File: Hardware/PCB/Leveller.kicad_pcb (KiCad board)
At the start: 2 copper layers, 20 x 48.2 mm, 41 parts, among them J13 Audio to Daisy, connect to J13, J14 Audio from Daisy, connect to 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, J17 Audio output, connect to J16, J18 Audio input, connect to J15, J6 Eurorack_Power, U1 TL074, U2 TL074

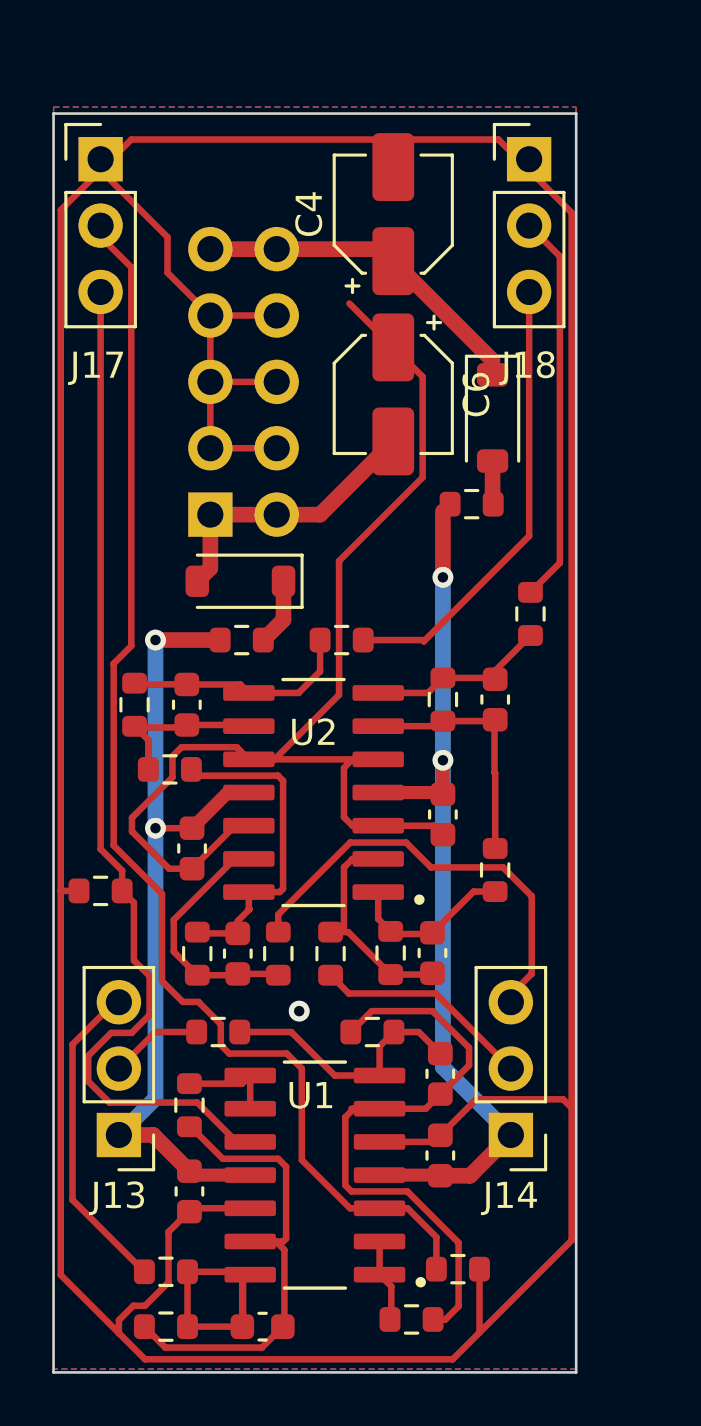
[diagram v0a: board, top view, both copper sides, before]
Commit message: HW 1.0c
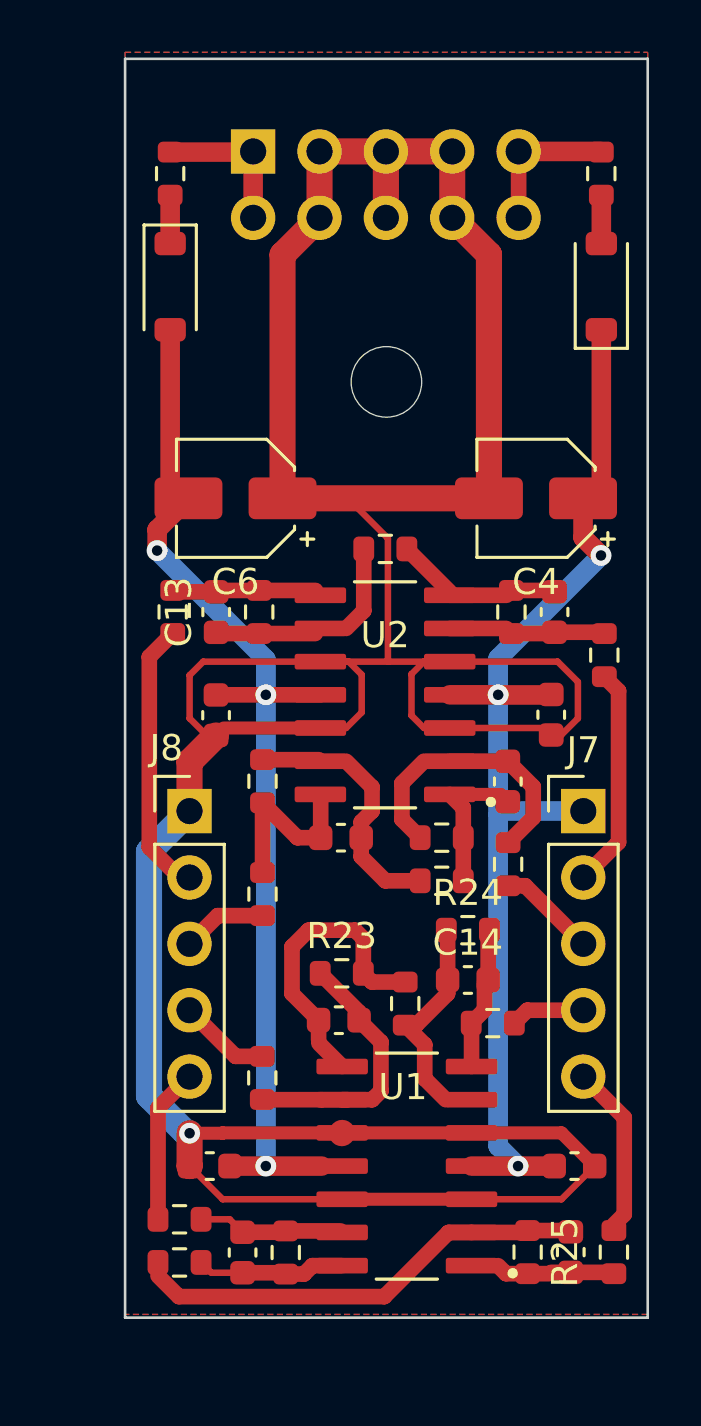
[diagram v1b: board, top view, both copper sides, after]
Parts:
- removed J13: Audio to Daisy, connect to J13, Connector_PinHeader_2.54mm:PinHeader_1x03_P2.54mm_Vertical
- removed J14: Audio from Daisy, connect to J10, Connector_PinHeader_2.54mm:PinHeader_1x03_P2.54mm_Vertical
- removed J17: Audio output, connect to J16, Connector_PinHeader_2.54mm:PinHeader_1x03_P2.54mm_Vertical
- removed J18: Audio input, connect to J15, Connector_PinHeader_2.54mm:PinHeader_1x03_P2.54mm_Vertical
- removed R11: 10K, Resistor_SMD:R_0603_1608Metric
- added C13: 560pF, Capacitor_SMD:C_0603_1608Metric, F.Cu at (58.2, 59.1)
- added C14: 47pF, Capacitor_SMD:C_0603_1608Metric, F.Cu at (67.9, 73.2)
- added J7: Conn_01x05, Connector_PinHeader_2.54mm:PinHeader_1x05_P2.54mm_Vertical, F.Cu at (72.3, 66.7)
- added J8: Conn_01x05, Connector_PinHeader_2.54mm:PinHeader_1x05_P2.54mm_Vertical, F.Cu at (57.2, 66.7)
- added MOUNT1: MountingHole_2.7mm_M2.5, MountingHole:MountingHole_2.7mm_M2.5, F.Cu at (64.7, 50.3)
- added R23: 100K, Resistor_SMD:R_0603_1608Metric, F.Cu at (63.0, 72.9)
- added R24: 100K, Resistor_SMD:R_0603_1608Metric, F.Cu at (67.9, 71.3)
- added R25: 100K, Resistor_SMD:R_0603_1608Metric, F.Cu at (70.1, 83.6)
- C2: value 560pF -> 47pF
- R5: value 2M -> 10K
- R9: value 2M -> 100K
- moved C9 21.1 mm to (59.2, 83.6), turned to 90 degrees
- moved C3 18.9 mm to (63.0, 67.7)
- moved FB1 18.1 mm to (56.5, 42.3), turned to -90 degrees
- moved R12 17.2 mm to (73.4, 83.6), turned to 90 degrees
- moved R9 15.5 mm to (60.9, 83.6), turned to -90 degrees
- moved R18 15.5 mm to (69.4, 68.8)
- moved J6 14.0 mm to (59.6, 41.5), turned to -90 degrees
- moved C7 13.9 mm to (71.2, 59.1)
- moved R13 13.8 mm to (69.5, 59.1)
- moved R16 13.7 mm to (56.6, 59.1), turned to 90 degrees
- moved C8 13.7 mm to (62.9, 74.7), turned to 180 degrees
- moved FB2 13.6 mm to (73.0, 42.3), turned to -90 degrees
- moved R14 13.4 mm to (59.9, 59.1)
- moved R15 13.0 mm to (64.7, 56.7), turned to 0 degrees
- moved C10 12.3 mm to (69.4, 65.6), turned to 90 degrees
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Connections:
- C10 pad 2: Net-(U2D--) -> Net-(U2A--)
- C2 pad 1: Net-(U1B--) -> (no net)
- C2 pad 2: Net-(C2-Pad2) -> Net-(U1A--)
- C3 pad 1: Net-(U1D--) -> Net-(U2D--)
- C4 pad 1: (no net) -> +12V
- C6 pad 2: (no net) -> -12V
- C7 pad 1: Net-(U2A--) -> Net-(U2B--)
- C8 pad 1: Net-(C8-Pad1) -> Net-(U1C--)
- C8 pad 2: Net-(U2B--) -> (no net)
- C9 pad 2: Net-(U2C--) -> Net-(U1D--)
- D1 pad 2: (no net) -> -12V
- D4 pad 1: (no net) -> +12V
- FB1 pad 1: -12V -> (no net)
- FB2 pad 1: +12V -> (no net)
- R10 pad 1: Net-(U1C--) -> Net-(C9-Pad1)
- R10 pad 2: Net-(U1D--) -> Net-(U1A--)
- R12 pad 1: Net-(C3-Pad2) -> (no net)
- R13 pad 1: Net-(U2A--) -> Net-(U2B--)
- R14 pad 1: Net-(U2A--) -> (no net)
- R14 pad 2: (no net) -> Net-(U2C--)
- R15 pad 1: Net-(U2B--) -> Net-(U2C--)
- R16 pad 2: Net-(C8-Pad1) -> (no net)
- R17 pad 1: Net-(C8-Pad1) -> Net-(U2B--)
- R17 pad 2: Net-(U2B--) -> (no net)
- R18 pad 1: Net-(C9-Pad1) -> Net-(U2A--)
- R18 pad 2: Net-(U2C--) -> (no net)
- R19 pad 2: Net-(U2D--) -> Net-(U2A--)
- R20 pad 1: Net-(U2C--) -> Net-(U2D--)
- R21 pad 1: Net-(U2D--) -> Net-(C3-Pad2)
- R21 pad 2: (no net) -> Net-(U2D--)
- R22 pad 2: Net-(C9-Pad1) -> Net-(C3-Pad2)
- R5 pad 1: (no net) -> Net-(U1D--)
- R5 pad 2: GND -> (no net)
- R6 pad 1: Net-(U1A--) -> (no net)
- R7 pad 1: Net-(U1B--) -> (no net)
- R7 pad 2: Net-(C2-Pad2) -> Net-(U1C--)
- R8 pad 1: Net-(C2-Pad2) -> (no net)
- R9 pad 1: (no net) -> Net-(U1D--)
- R9 pad 2: GND -> Net-(C9-Pad1)
- U1 pad 1: Net-(U1A--) -> (no net)
- U1 pad 10: (no net) -> GND
- U1 pad 14: Net-(C3-Pad2) -> Net-(C9-Pad1)
- U1 pad 3: (no net) -> GND
- U1 pad 7: Net-(C2-Pad2) -> (no net)
- U1 pad 8: Net-(U1C--) -> (no net)
- U2 pad 1: Net-(C7-Pad2) -> Net-(C10-Pad1)
- U2 pad 14: Net-(C10-Pad1) -> Net-(C3-Pad2)
- U2 pad 7: Net-(C8-Pad1) -> Net-(C7-Pad2)
- U2 pad 8: Net-(C9-Pad1) -> (no net)
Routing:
- net (no net): track 188.0 -> 87.1 mm
- net GND: track 210.4 -> 141.0 mm
- net Net-(U1B--): track 24.2 -> 8.98 mm
- net Net-(U1A--): track 3.45 -> 17.0 mm
- net Net-(U1D--): track 18.7 -> 5.50 mm
- net -12V: track 30.6 -> 42.0 mm, vias 2 -> 3
- net Net-(C2-Pad2): track 10.0 -> 0.00 mm
- net +12V: track 34.9 -> 44.9 mm, vias 2 -> 3
- net Net-(U1C--): track 3.72 -> 10.3 mm
- net Net-(C8-Pad1): track 6.57 -> 0.00 mm
- net Net-(C10-Pad1): track 12.1 -> 5.86 mm
- net Net-(U2B--): track 9.14 -> 5.62 mm
- net Net-(C9-Pad1): track 8.73 -> 5.64 mm
- net Net-(C3-Pad2): track 9.65 -> 7.09 mm
- net Net-(U2A--): track 8.26 -> 10.7 mm
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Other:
- board text added: "Loop v1.0c"
- board text removed: "Loop v1.0b"
